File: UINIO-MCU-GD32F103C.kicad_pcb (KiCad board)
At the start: 2 copper layers, 68.4 x 20.3 mm, 41 parts, among them J1 Conn_01x24_Pin, J2 Conn_01x24_Pin, J3 Conn_01x04_Pin, SW1 BOOT1, SW2 NRST, SW3 BOOT0, U1 ME6211C33M5G-N, U2 GD32F103C8T6, Y1 32.768KHz, Y2 8MHz

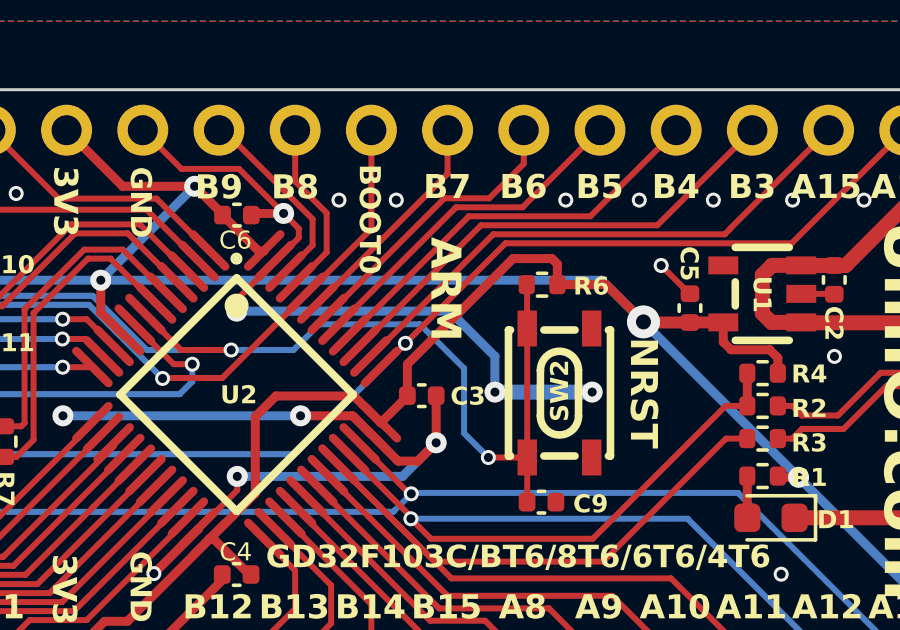
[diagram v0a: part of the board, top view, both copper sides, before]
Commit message: Release UINIO-MCU-GD32F103C version 2.0.0.
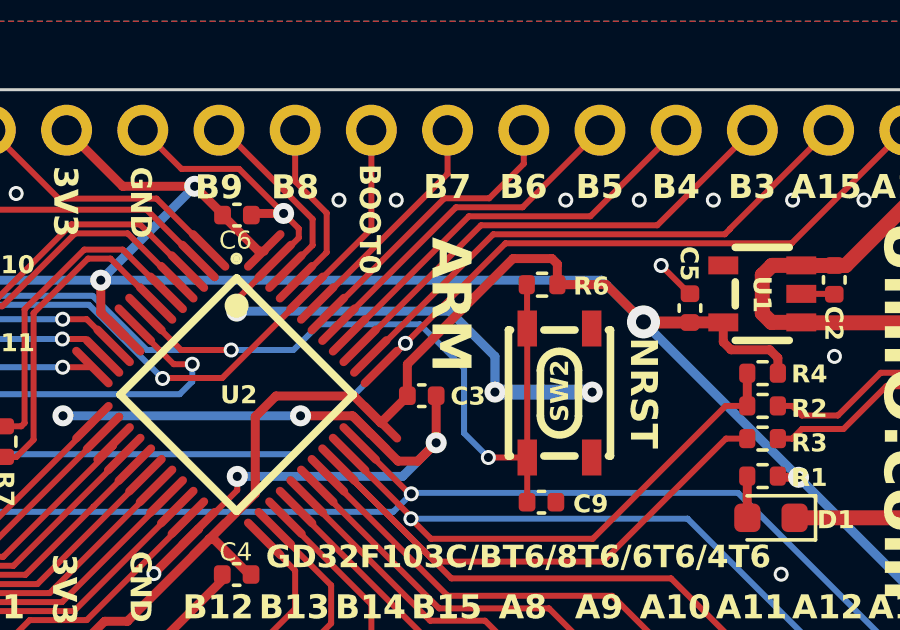
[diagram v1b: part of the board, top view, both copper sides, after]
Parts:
- moved ? 0.46 mm to (140.1, 100.7)
